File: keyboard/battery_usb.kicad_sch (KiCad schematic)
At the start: 11 parts, among them SW1 SW_DIP_x01, U2 USB2514-HZH (C184347), U3 TPS62140

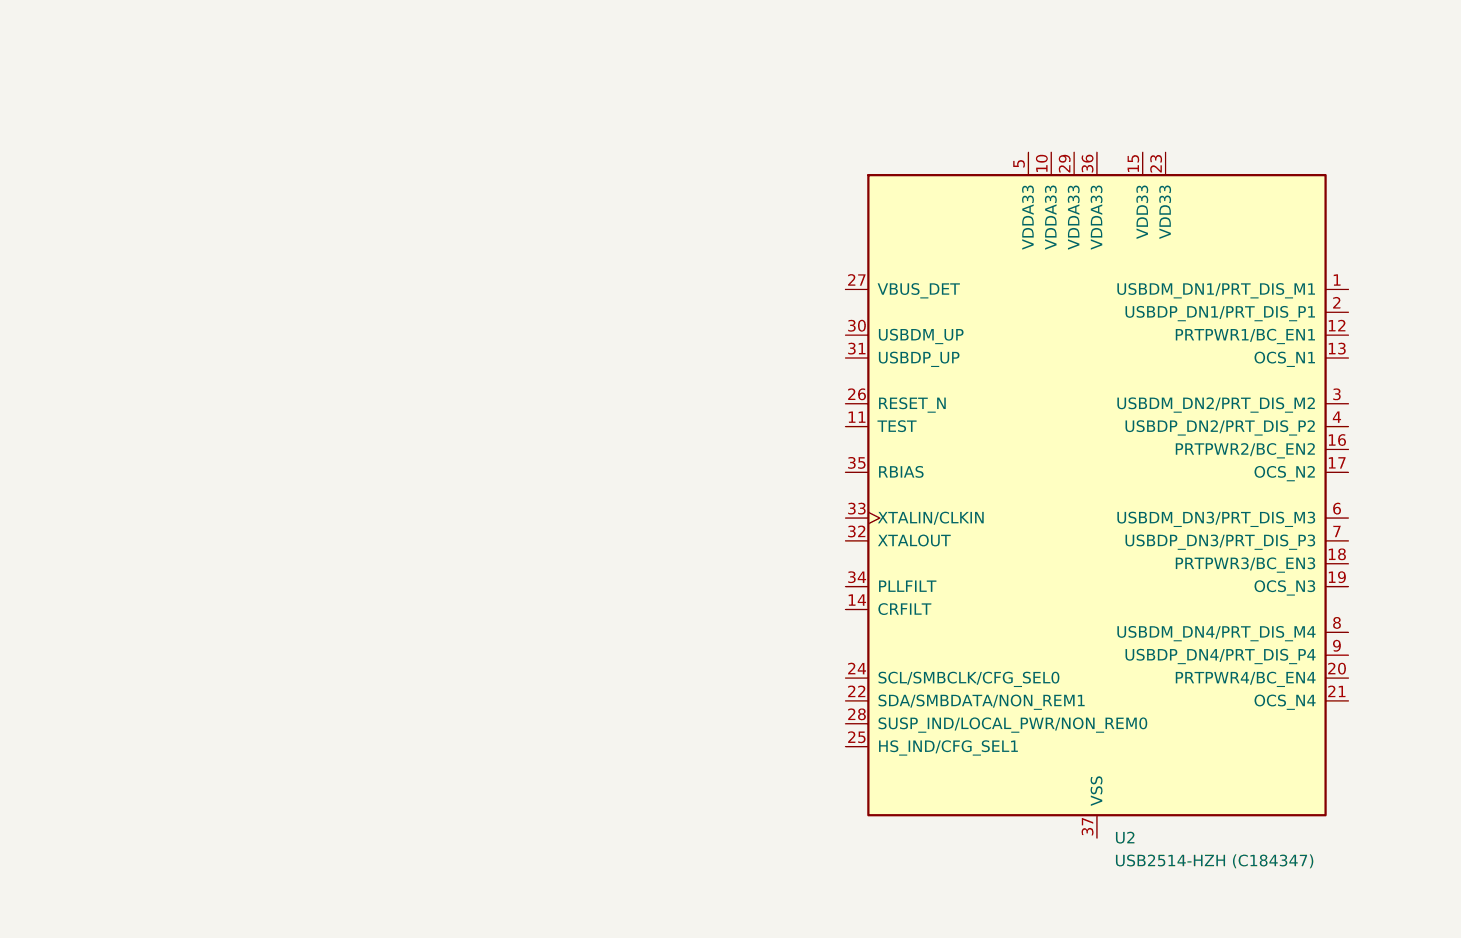
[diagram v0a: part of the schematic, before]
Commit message: wireing
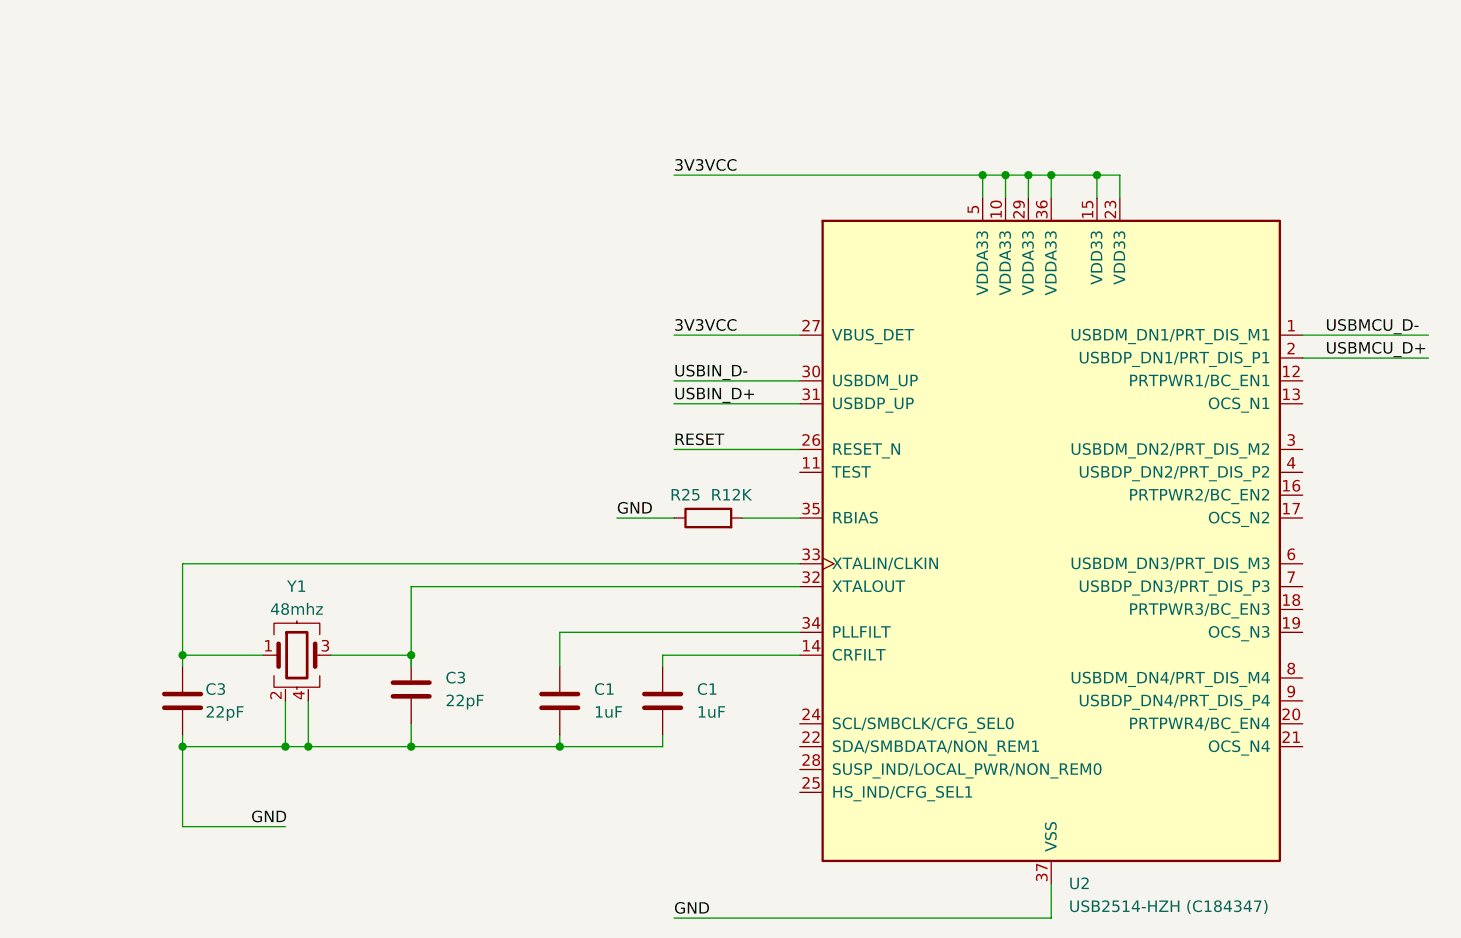
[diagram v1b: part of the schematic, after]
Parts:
- added C1 (x2): 1uF, Capacitor_SMD:C_0402_1005Metric, symbol Device:C
- added C3 (x2): 22pF, Capacitor_SMD:C_0402_1005Metric, symbol Device:C
- added R25: R12K, symbol Device:R
- added Y1: 48mhz, Crystal:Crystal_SMD_TXC_7M-4Pin_3.2x2.5mm, symbol Device:Crystal_GND24
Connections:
- net 3V3VCC: now also U2.10 (VDDA33), U2.15 (VDD33), U2.23 (VDD33), U2.27 (VBUS_DET), U2.29 (VDDA33), U2.36 (VDDA33), U2.5 (VDDA33)
- net GND: now also U2.37 (VSS), C1.2, C1.2, C3.2, C3.2, R25.1, Y1.2, Y1.4
- net USBMCU_D-: now reaches U2.1 (USBDM_DN1/PRT_DIS_M1)
- net at U2.14 (CRFILT): now also C1.1
- net USBMCU_D+: now reaches U2.2 (USBDP_DN1/PRT_DIS_P1)
- net RESET: now reaches U2.26 (RESET_N)
- net USBIN_D-: now reaches U2.30 (USBDM_UP)
- net USBIN_D+: now reaches U2.31 (USBDP_UP)
- net at U2.32 (XTALOUT): now also C3.1, Y1.3
- net at U2.33 (XTALIN/CLKIN): now also C3.1, Y1.1
- net at U2.34 (PLLFILT): now also C1.1
- net at U2.35 (RBIAS): now also R25.2
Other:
- moved on the sheet: U2

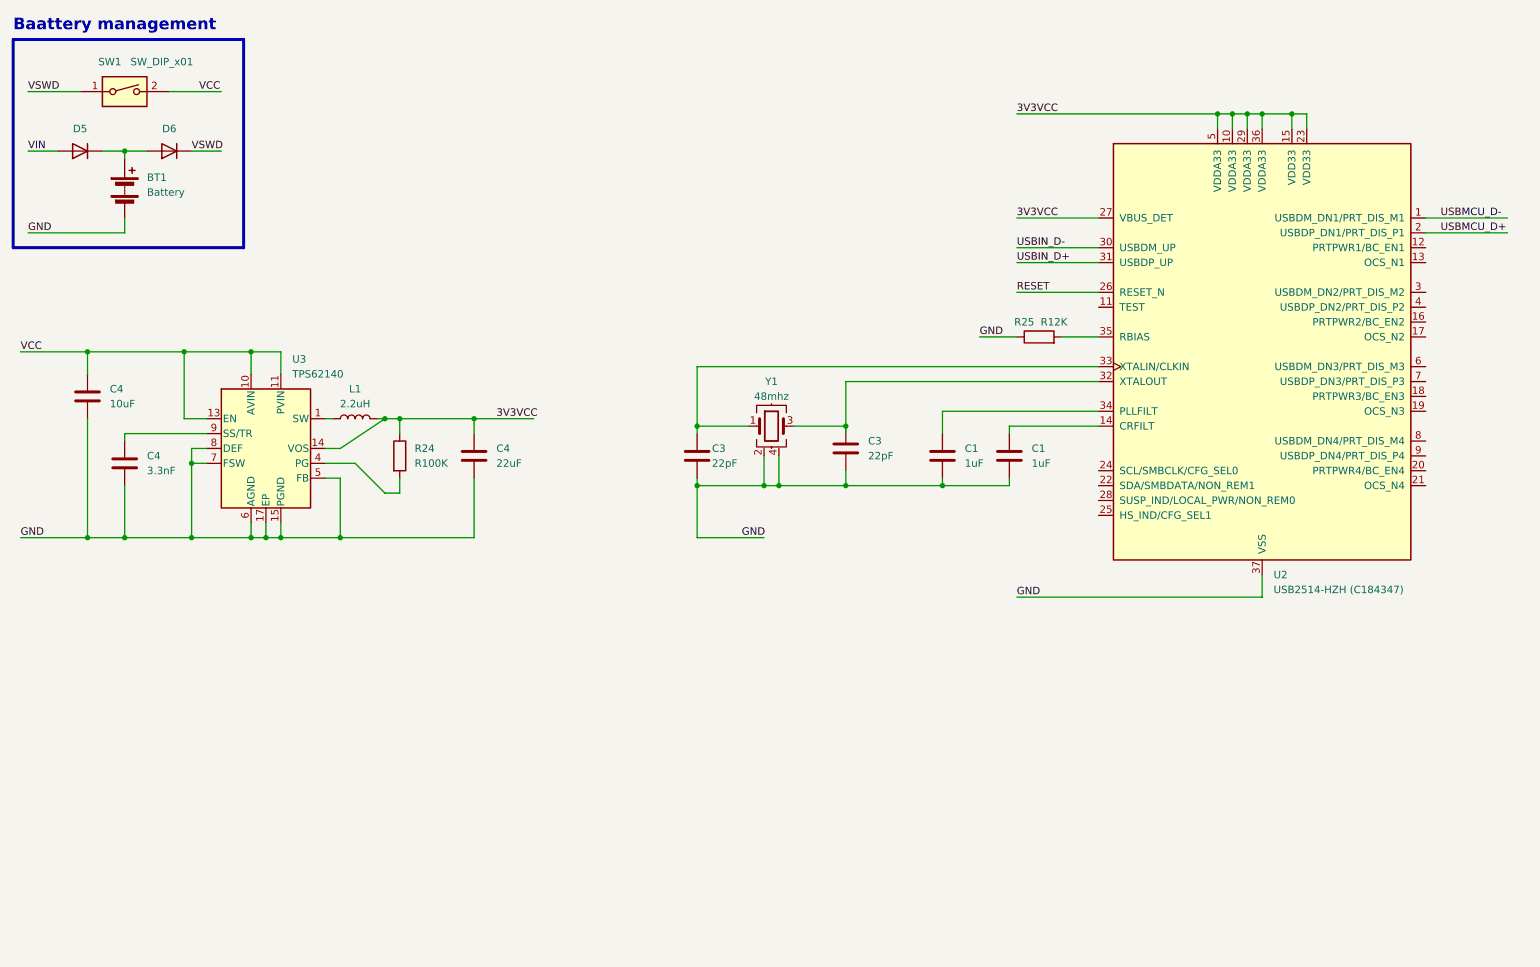
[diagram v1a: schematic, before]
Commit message: usb hub wireing half
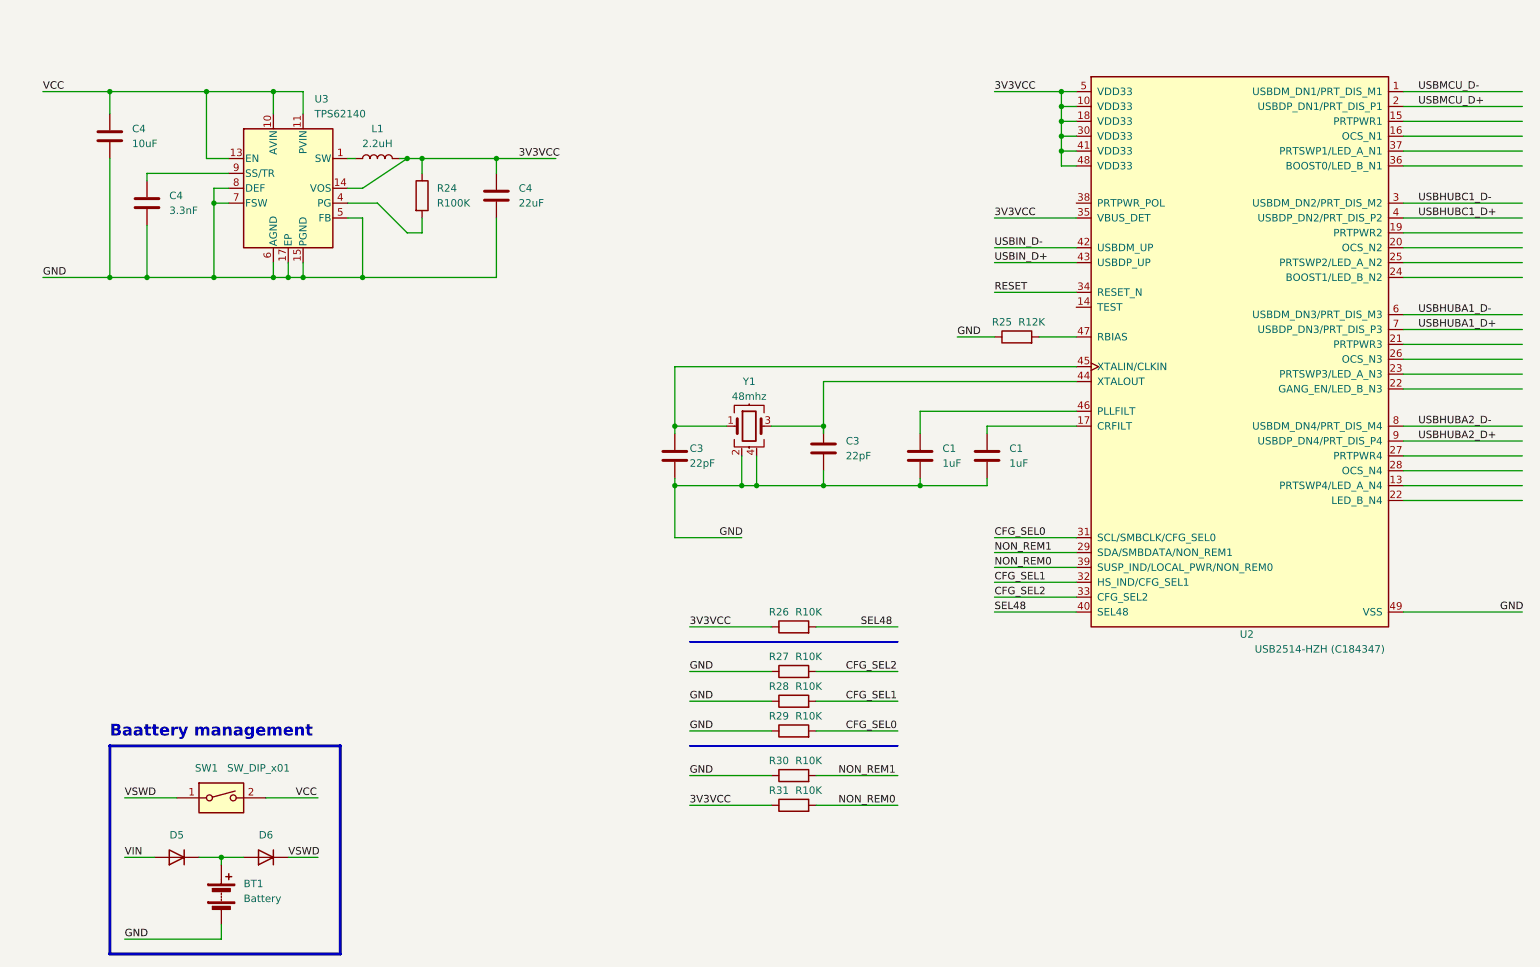
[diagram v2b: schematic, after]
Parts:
- added R26, R27, R28, R29, R30, R31: R10K, symbol Device:R
- U2: footprint Package_DFN_QFN:VQFN-48-1EP_7x7mm_P0.5mm_EP4.1x4.1mm -> Package_DFN_QFN:VQFN-48-1EP_7x7mm_P0.5mm_EP4.1x4.1mm_ThermalVias
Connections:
- net 3V3VCC: now also U2.18 (VDD33), U2.30 (VDD33), U2.35 (VBUS_DET), U2.41 (VDD33), U2.48 (VDD33), R26.1, R31.1; no longer U2.15 (VDD33), U2.23 (VDD33), U2.27 (VBUS_DET), U2.29 (VDDA33), U2.36 (VDDA33)
- net GND: now also U2.49 (VSS), R27.1, R28.1, R29.1, R30.1; no longer U2.37 (VSS)
- net RESET: now also U2.34 (RESET_N); no longer U2.26 (RESET_N)
- net USBIN_D+: now also U2.43 (USBDP_UP); no longer U2.31 (USBDP_UP)
- net USBIN_D-: now also U2.42 (USBDM_UP); no longer U2.30 (USBDM_UP)
- net at U2.14 (TEST): no longer C1.1
- net at U2.17 (CRFILT): now also C1.1
- net USBHUBC1_D-: now reaches U2.3 (USBDM_DN2/PRT_DIS_M2)
- net at C3.1, Y1.3: now also U2.44 (XTALOUT); no longer U2.32 (XTALOUT)
- net at C3.1, Y1.1: now also U2.45 (XTALIN/CLKIN); no longer U2.33 (XTALIN/CLKIN)
- net at C1.1: now also U2.46 (PLLFILT); no longer U2.34 (PLLFILT)
- net at R25.2: now also U2.47 (RBIAS); no longer U2.35 (RBIAS)
- net USBHUBC1_D+: now reaches U2.4 (USBDP_DN2/PRT_DIS_P2)
- net USBHUBA1_D-: now reaches U2.6 (USBDM_DN3/PRT_DIS_M3)
- net USBHUBA1_D+: now reaches U2.7 (USBDP_DN3/PRT_DIS_P3)
- net USBHUBA2_D-: now reaches U2.8 (USBDM_DN4/PRT_DIS_M4)
- net USBHUBA2_D+: now reaches U2.9 (USBDP_DN4/PRT_DIS_P4)
- new net CFG_SEL0: R29.2, U2.31 (SCL/SMBCLK/CFG_SEL0)
- new net CFG_SEL1: R28.2, U2.32 (HS_IND/CFG_SEL1)
- new net CFG_SEL2: R27.2, U2.33 (CFG_SEL2)
- new net NON_REM0: R31.2, U2.39 (SUSP_IND/LOCAL_PWR/NON_REM0)
- new net NON_REM1: R30.2, U2.29 (SDA/SMBDATA/NON_REM1)
- new net SEL48: R26.2, U2.40 (SEL48)
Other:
- moved on the sheet: BT1, C1, C3, C4, D5, D6, L1, R24, R25, SW1, U3, Y1
